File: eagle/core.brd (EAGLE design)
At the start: 100.3 x 21.6 mm, 29 parts, among them K1 AQH2223A, SW0 TPTP10R, SW1 TPTP10R

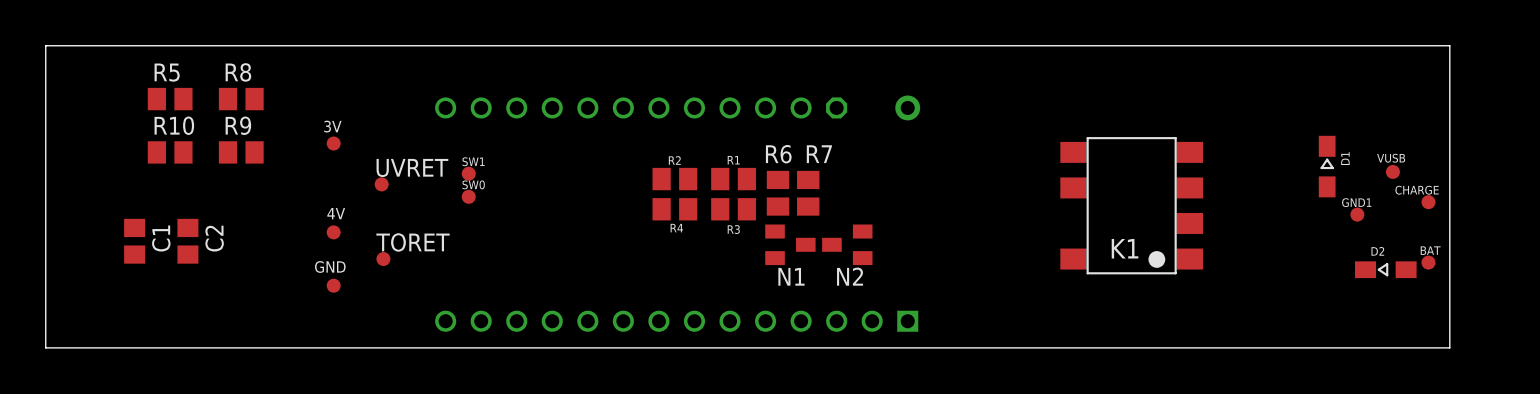
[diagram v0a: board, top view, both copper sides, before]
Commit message: ffc breakout and core changes
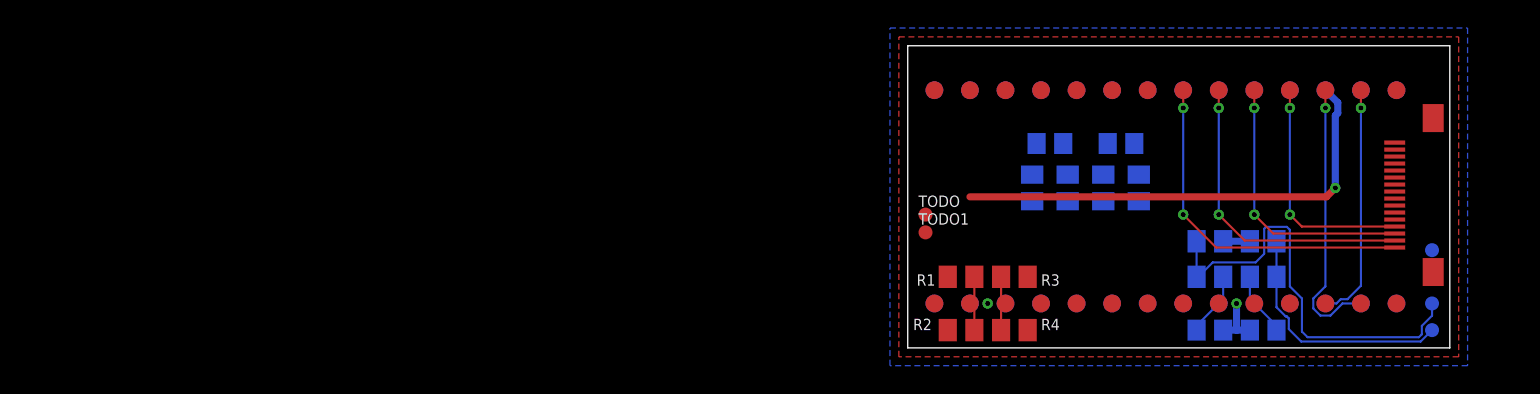
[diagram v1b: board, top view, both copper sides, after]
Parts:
- removed 3V, 4V, BAT, CHARGE, GND, GND1, SW0, SW1, TORET, UVRET, VUSB: TPTP10R, testpad:TP10R
- removed D1, D2: 1N5817WS, general:SOD323-W
- removed K1: AQH2223A, relay:DIL07SMD
- removed N1, N2: BC846, transistor:SOT23
- added C3, C4: 10u, resistor:C0805
- added ENCL, ENCR, MBTN, SBTN, TODO, TODO1: TPTP10R, testpad:TP10R
- added R11, R12: 10k, resistor:M0805
- added U$2: TEENSYSMALL, general:TEENSYSMALL
- added U$3: 16PINFFC, general:16PINFFC
- R1, R2, R3, R4: value 100k -> 20M
- R6, R7: value 1k -> 10k
- R8, R9: value 100k -> 10k
- U$1: value TEENSY40EDGES -> TEENSY4; device general:TEENSY40 -> general:TEENSYSMALL
- moved C1 80.9 mm to (87.0, 1.27), flipped to the bottom, turned to 0 degrees
- moved R5 79.1 mm to (87.0, 5.08), flipped to the bottom, turned to 180 degrees
- moved R10 74.8 mm to (83.2, 5.08), flipped to the bottom
- moved R8 73.7 mm to (87.0, 7.62), flipped to the bottom
- moved C2 73.3 mm to (83.2, 1.27), flipped to the bottom, turned to 180 degrees
- moved R9 69.5 mm to (83.2, 7.62), flipped to the bottom, turned to 180 degrees
- moved U$1 36.2 mm to (81.3, 10.8), flipped to the top, turned to 180 degrees
- moved R4 25.7 mm to (69.2, 1.27), turned to 180 degrees
- moved R2 23.1 mm to (65.4, 1.27)
- moved R6 20.7 mm to (73.0, 11.4), flipped to the bottom
- moved R3 20.6 mm to (69.2, 5.08), turned to 0 degrees
- moved R1 17.7 mm to (65.4, 5.08)
- moved R7 16.0 mm to (70.5, 11.4), flipped to the bottom, turned to 270 degrees
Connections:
- removed net N$1: K1.2
- removed net N$10: N1.1, R6.1
- removed net N$11: N2.1, R7.1
- removed net N$12: N1.2, UVRET.TP
- removed net N$13: N2.2, TORET.TP
- removed net N$2: R3.2, R4.2, U$1.21-A7/RX5/BCLK1
- removed net N$4: BAT.TP, D2.A
- removed net N$5: D2.C, K1.8
- removed net N$6: R1.2, R2.2, U$1.20-A6/TX5/LRCLK1
- removed net N$7: K1.3
- removed net N$8: R7.2, U$1.23-A9/CRX1/CCLK1
- removed net N$9: R6.2, U$1.22-A8/CTX1
- removed net VUSB: CHARGE.TP, D1.A, R1.1, VUSB.TP
- new net ANTT1: R1.1, R2.2, U$1.14
- new net ANTT2: R3.1, R4.2, U$1.15
- new net BCLK: U$3.12
- new net DC: U$3.5
- new net DOUT: U$3.11
- new net LRCL: U$3.10
- new net MBTN: MBTN.TP, R11.1, R12.2
- new net MBTNPIN: C4.1, R12.1, TODO.TP
- new net MOSI: U$3.3
- new net PWM1: U$1.5, U$3.16
- new net PWM2: U$1.4, U$3.15
- new net PWM3: U$1.3, U$3.14
- new net PWM4: U$1.2, U$3.13
- new net SBTN: R6.1, R7.2, SBTN.TP
- new net SBTNPIN: C3.1, R7.1, TODO1.TP
- new net SCK: U$3.4
- new net SSCL: U$3.2
- new net SSDA: U$3.1
- new net T4RX: U$1.0, U$2.1
- new net T4TX: U$1.1, U$2.0
- new net TFTCS: U$3.7
- new net TFTRST: U$3.6
- net 3V: now also R1.2, R11.2, R3.2, R6.2, U$1.3V, U$2.3V; no longer 3V.TP, N1.3, N2.3, U$1.3V3-1
- net 4V: no longer 4V.TP, D1.C, K1.6, R3.1
- net ENCL: now also ENCL.TP
- net ENCPINL: now also U$2.3
- net ENCPINR: now also U$2.4
- net ENCR: now also ENCR.TP
- net GND: now also C3.2, C4.2, U$1.GND, U$2.GND, U$3.BASE1, U$3.BASE2; no longer GND.TP, GND1.TP, U$1.GND1
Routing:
- net 3V: track 0.00 -> 35.7 mm, vias 0 -> 1
- net ENCR: track 0.00 -> 30.8 mm
- net PWM1: track 0.00 -> 25.0 mm, vias 0 -> 2
- net PWM2: track 0.00 -> 22.2 mm, vias 0 -> 2
- net T4TX: track 0.00 -> 19.9 mm, vias 0 -> 1
- net PWM3: track 0.00 -> 19.5 mm, vias 0 -> 2
- net ENCL: track 0.00 -> 17.6 mm
- net T4RX: track 0.00 -> 17.0 mm, vias 0 -> 1
- net PWM4: track 0.00 -> 16.7 mm, vias 0 -> 2
- net ENCPINR: track 0.00 -> 4.60 mm
- net ENCPINL: track 0.00 -> 4.60 mm
- net ANTT2: track 0.00 -> 4.07 mm
- net ANTT1: track 0.00 -> 4.07 mm
- net GND: track 0.00 -> 3.81 mm, vias 0 -> 2
- added copper zone on layer 1, net GND
- added copper zone on layer 16, net GND
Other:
- board size 100.3 x 21.6 mm -> 38.7 x 21.6 mm

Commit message: mini probe
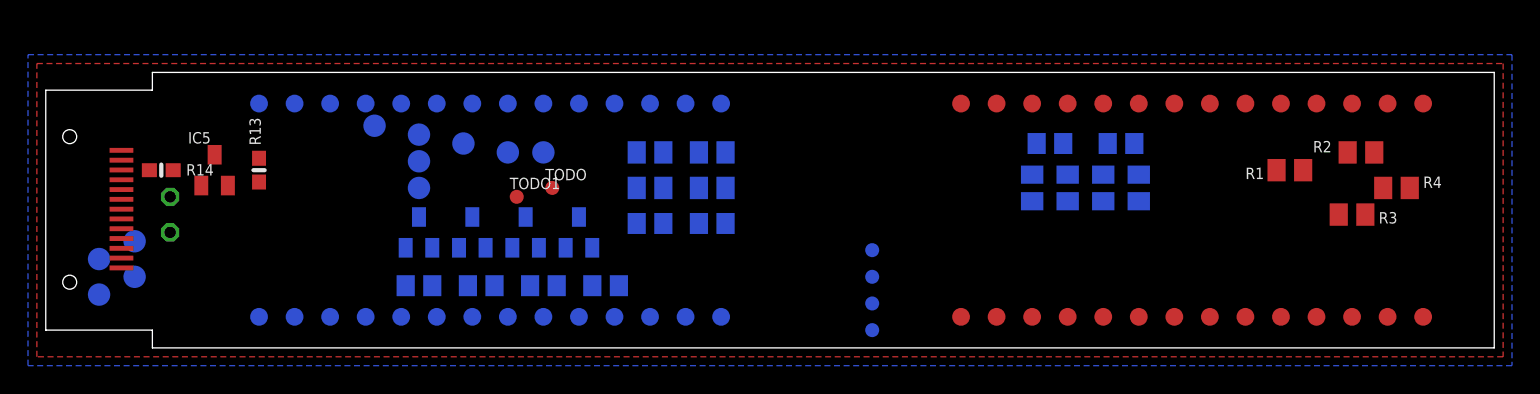
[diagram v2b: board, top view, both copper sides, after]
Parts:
- removed U$3: 16PINFFC, general:16PINFFC
- added 3V, BCLK, DOUT, GND, L1-, L2-, L3-, L4-, LRCL, SSCL, SSDA: TPTP16R, testpad:TP16R
- added IC5: APX803, adafruit:SOT23
- added LED1: (no value), led:LED3MM
- added R13: 10K, microbuilder:0603-NO
- added R14: 22, microbuilder:0603-NO
- added R15, R16, R17, R18: (no value), resistor:R0805
- added T1, T2, T3, T4: BC846, transistor:SOT23
- added U$4: TFT, general:MICROBUILDER_TFT_1.14IN_240X135_WRAPUNDER
- moved U$1 48.3 mm to (33.0, 9.84), flipped to the bottom, turned to 0 degrees
- moved C2 40.7 mm to (43.2, 8.89), turned to 0 degrees
- moved R10 40.5 mm to (43.2, 11.4)
- moved R9 40.5 mm to (43.2, 14.0)
- moved C1 40.1 mm to (47.6, 8.89), turned to 180 degrees
- moved ENCL 40.0 mm to (59.1, 1.27)
- moved ENCR 40.0 mm to (59.1, 3.17)
- moved MBTN 40.0 mm to (59.1, 5.08)
- moved SBTN 40.0 mm to (59.1, 6.99)
- moved R5 39.9 mm to (47.6, 11.4)
- moved R8 39.9 mm to (47.6, 14.0)
- moved R2 31.3 mm to (94.0, 14.0)
- moved TODO1 29.3 mm to (33.7, 10.8)
- moved R4 29.1 mm to (96.5, 11.4)
- moved TODO 26.7 mm to (36.2, 11.4)
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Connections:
- new net !TFTRST: IC5.2, R13.1
- new net L1-: L1-.TP, T1.3
- new net L2-: L2-.TP, T2.3
- new net L3-: L3-.TP, T3.3
- new net L4-: L4-.TP, LED1.K, T4.3
- new net N$1: R14.2, U$4.11
- new net N$2: R15.2, T1.1
- new net N$3: R16.2, T2.1
- new net N$4: R17.2, T3.1
- new net N$5: R18.2, T4.1
- net 3V: now also 3V.TP, IC5.3, LED1.A, R13.2, U$4.10, U$4.12
- net BCLK: now also BCLK.TP; no longer U$3.12
- net DC: now also U$1.9, U$4.5; no longer U$3.5
- net DOUT: now also DOUT.TP; no longer U$3.11
- net GND: now also GND.TP, IC5.1, R14.1, T1.2, T2.2, T3.2, T4.2, U$4.13, U$4.8; no longer U$3.BASE1, U$3.BASE2
- net LRCL: now also LRCL.TP; no longer U$3.10
- net MOSI: now also U$1.11, U$4.3; no longer U$3.3
- net PWM1: now also R15.1; no longer U$3.16
- net PWM2: now also R16.1; no longer U$3.15
- net PWM3: now also R17.1; no longer U$3.14
- net PWM4: now also R18.1; no longer U$3.13
- net SCK: now also U$1.13, U$4.4; no longer U$3.4
- net SSCL: now also SSCL.TP; no longer U$3.2
- net SSDA: now also SSDA.TP; no longer U$3.1
- net TFTCS: now also U$1.10, U$4.7; no longer U$3.7
- net TFTRST: now also U$1.7, U$4.6; no longer U$3.6
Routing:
- net 3V: track 35.7 -> 0.00 mm, vias 1 -> 0
- net ENCR: track 30.8 -> 0.00 mm
- net PWM1: track 25.0 -> 0.00 mm, vias 2 -> 0
- net PWM2: track 22.2 -> 0.00 mm, vias 2 -> 0
- net T4TX: track 19.9 -> 0.00 mm, vias 1 -> 0
- net PWM3: track 19.5 -> 0.00 mm, vias 2 -> 0
- net ENCL: track 17.6 -> 0.00 mm
- net T4RX: track 17.0 -> 0.00 mm, vias 1 -> 0
- net PWM4: track 16.7 -> 0.00 mm, vias 2 -> 0
- net ENCPINR: track 4.60 -> 0.00 mm
- net ENCPINL: track 4.60 -> 0.00 mm
- net ANTT2: track 4.07 -> 0.00 mm
- net ANTT1: track 4.07 -> 0.00 mm
- net GND: track 3.81 -> 0.00 mm, vias 2 -> 0
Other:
- board size 38.7 x 21.6 mm -> 103.5 x 19.7 mm
